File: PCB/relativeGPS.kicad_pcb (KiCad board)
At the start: 2 copper layers, 60 x 60 mm, 90 parts, among them CN1 FTSH-107-01-L-DV-K-P-TR, CN2 Solder_Jumper-2_Open, CN3 TC2030-IDC, CN4 5033981892, IC1 MIC5330-SSYML-TR, SW1 switch_slide_2pos, SW2 EVQ-P7A01P, SW3 EVQ-P7A01P, U1 LSM303AH, U10 RYLR998, U11 74LVC1T45GW,125, U2 TCA39306DCUR, U3 BGA725L6E6327FTSA1, U4 ST1S12GR, U5 B39162B4327P810, U6 TESEO-LIV3R, U7 AAA_2X_Holder, U8 TPS61222DCKR, U9 TPS79318DBVR

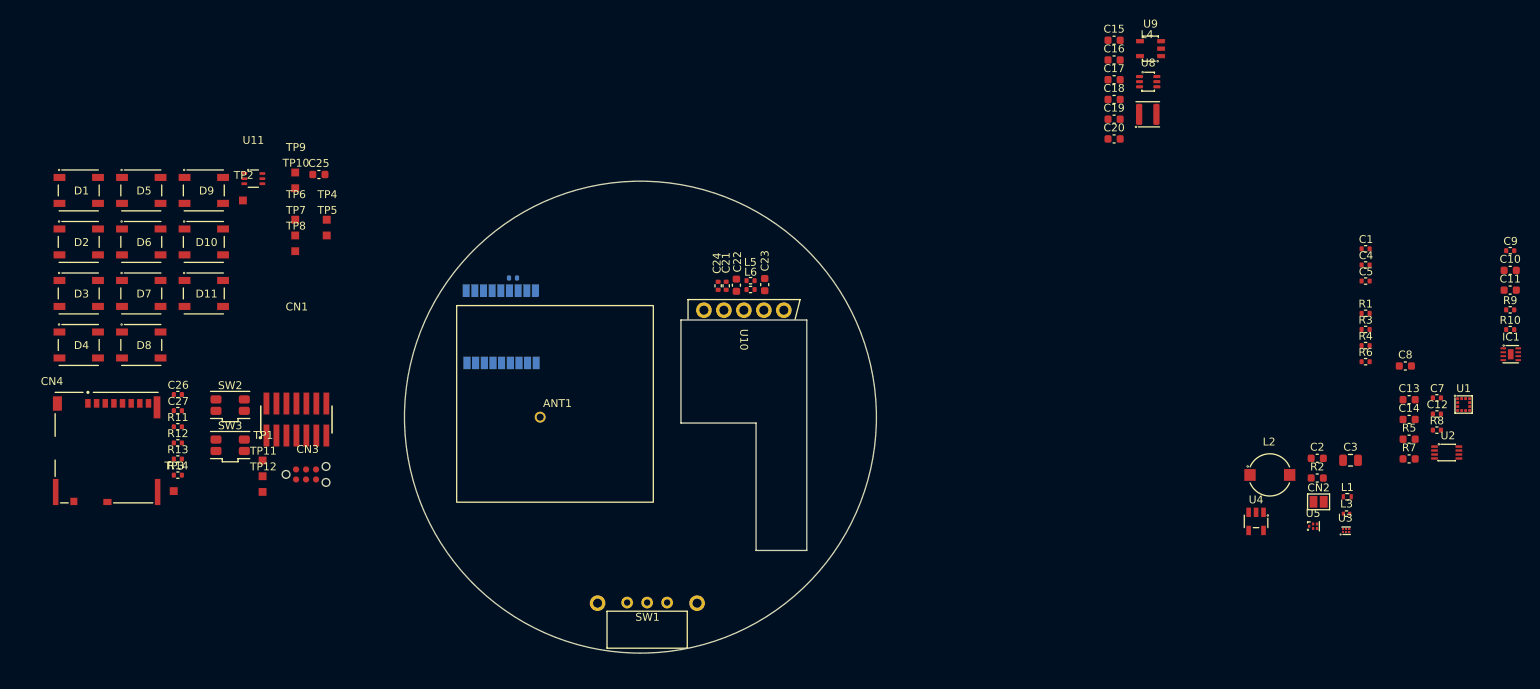
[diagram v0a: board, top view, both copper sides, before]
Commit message: Layout start
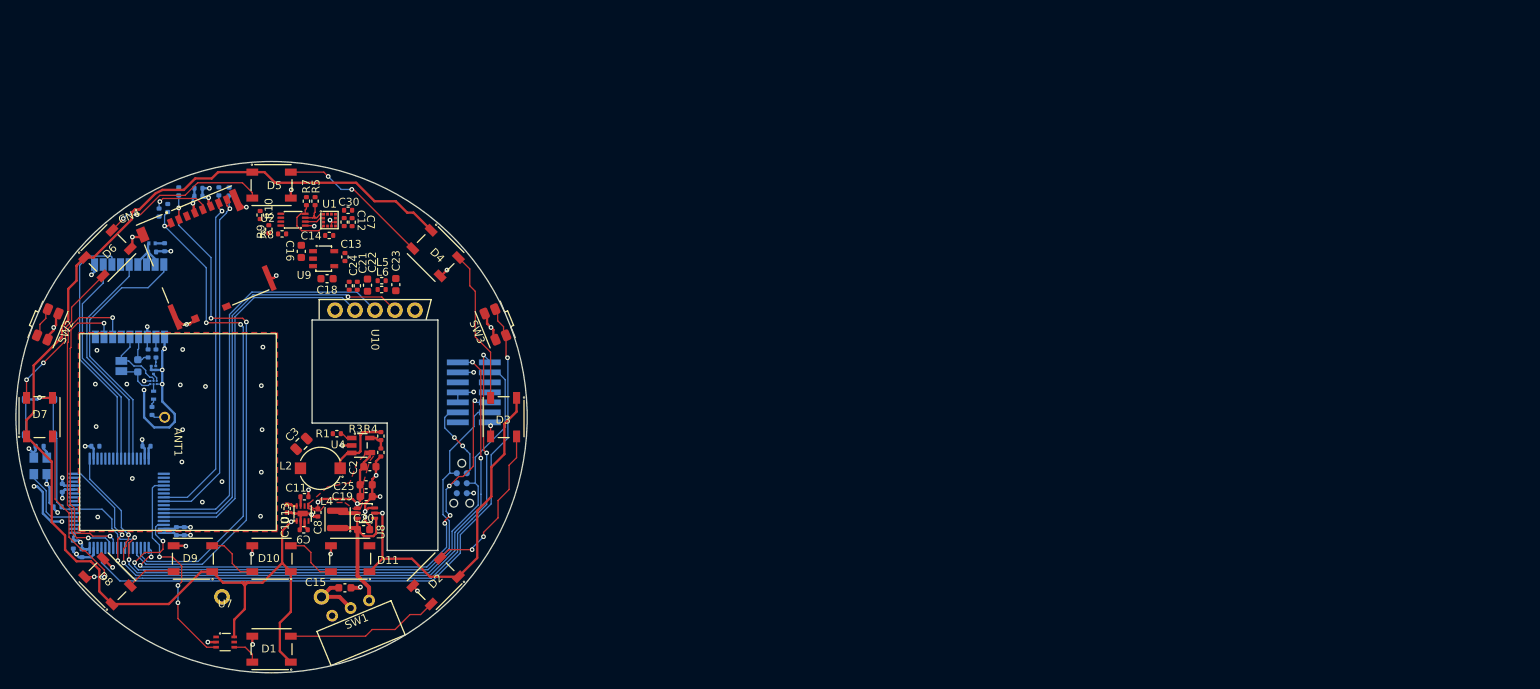
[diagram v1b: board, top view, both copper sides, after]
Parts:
- removed IC1: MIC5330-SSYML-TR, 004-Power:MIC5330
- removed TP1, TP10, TP11, TP12, TP2, TP3, TP4, TP5, TP6, TP7, TP8, TP9: TP_square_1mm, 011-Misc:Testpoint_square_1mm
- added B7: AAA_2X_Holder, 004-Power:AAA_2X_Holder, B.Cu at (100.0, 99.2)
- added C28: C_10nF_50V_10%_X7R_0402_H0.55, 002-Capacitors:C_0402_H0.55, B.Cu at (70.5, 103.7)
- added C29: C_100nF_50V_10%_X7R_0402_H0.55, 002-Capacitors:C_0402_H0.55, B.Cu at (72.8, 111.4)
- added C30: C_2.2uF_25V_25%_X5R_0402_H0.55, 002-Capacitors:C_0402_H0.55, F.Cu at (109.7, 73.7)
- added C31: C_100nF_50V_10%_X7R_0402_H0.55, 002-Capacitors:C_0402_H0.55, B.Cu at (74.8, 116.2)
- added C32: C_100nF_50V_10%_X7R_0402_H0.55, 002-Capacitors:C_0402_H0.55, B.Cu at (73.4, 109.0)
- added C33: C_100nF_50V_10%_X7R_0402_H0.55, 002-Capacitors:C_0402_H0.55, B.Cu at (77.6, 103.7)
- added C34: C_100nF_50V_10%_X7R_0402_H0.55, 002-Capacitors:C_0402_H0.55, B.Cu at (84.1, 103.7)
- added C35: C_100nF_50V_10%_X7R_0402_H0.55, 002-Capacitors:C_0402_H0.55, B.Cu at (87.9, 114.5)
- added C36: C_10uF_10V_20%_X5R_0402_H0.55, 002-Capacitors:C_0402_H0.55, B.Cu at (88.9, 114.5)
- added R15: R_0R_1%_1/16W_0402, 001-Resistors:R_0402_H0.4, B.Cu at (85.7, 74.0)
- added SW4: TL3315NF160Q, 009-Connectors:TL3315NF160Q, B.Cu at (70.5, 100.0)
- added U12: ASE-8.000MHZ-L-C-T, 005-ICs:ASE-8.000MHZ-L-C-T, B.Cu at (70.6, 106.2)
- added U13: MIC5330-SSYML-TR, 004-Power:MIC5330, F.Cu at (103.9, 112.3)
- C1, C26, C27, C4, C5, CN1, CN2, CN3, L1, L3, R11, R12, R13, R14, R2, R6, U3, U5: moved to B.Cu
- C10, C11, C8: value C_1uF_50V_10%_X5R_0603_H0.9 -> C_1uF_50V_10%_X5R_0402_H0.55; footprint 002-Capacitors:C_0603_H0.95 -> 002-Capacitors:C_0402_H0.55
- C13: value C_220nF_50V_10%_X7R_0603_H0.9 -> C_2.2uF_25V_25%_X5R_0402_H0.55; footprint 002-Capacitors:C_0603_H0.95 -> 002-Capacitors:C_0402_H0.55
- C14: value C_10uF_10V_20%_X5R_0603H0.9 -> C_220nF_16V_10%_X7R_0402_H0.55; footprint 002-Capacitors:C_0603_H0.95 -> 002-Capacitors:C_0402_H0.55
- C17: value C_10uF_10V_20%_X5R_0603H0.9 -> C_100nF_50V_10%_X7R_0402_H0.55; footprint 002-Capacitors:C_0603_H0.95 -> 002-Capacitors:C_0402_H0.55; moved to B.Cu
- R5, R7: value R_4k7_1%_1/10W_0603 -> R_4k7_5%_1/16W_0402; footprint 001-Resistors:R_0603_H0.55 -> 001-Resistors:R_0402_H0.4
- U11: value 74LVC1T45GW,125 -> STM32L431RCT6TR; footprint 005-ICs:TSSOP6_SOT363-2.step -> 007-MCUs:LQFP-64_10x10mm_P0.5mm; moved to B.Cu
- U7: value AAA_2X_Holder -> 74LVC1T45GW.125; footprint 004-Power:AAA_2X_Holder -> 005-ICs:TSSOP6_SOT363-2.step; moved to F.Cu
- moved R9 159.4 mm to (98.5, 74.3), turned to -90 degrees
- moved C10 158.4 mm to (102.0, 111.6), turned to -90 degrees
- moved R10 158.3 mm to (99.7, 76.1), turned to 90 degrees
- moved C9 157.4 mm to (104.1, 114.3), turned to 180 degrees
- moved L3 155.7 mm to (84.8, 77.9), turned to 180 degrees
- moved C1 155.7 mm to (84.8, 99.2), turned to 90 degrees
- moved C11 155.5 mm to (104.2, 110.1)
- moved R6 154.8 mm to (84.3, 91.9), turned to 90 degrees
- moved C4 154.2 mm to (85.3, 91.9), turned to 90 degrees
- moved CN2 153.2 mm to (80.9, 93.5), turned to -90 degrees
- moved U3 152.8 mm to (85.0, 95.6)
- moved C5 152.8 mm to (86.4, 78.4), turned to -90 degrees
- moved L1 152.3 mm to (85.0, 97.2), turned to 90 degrees
- moved R2 150.6 mm to (83.0, 93.5), turned to 90 degrees
- moved U2 149.6 mm to (102.7, 74.9), turned to 180 degrees
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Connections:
- C11 pad 1: +3.3V -> +3.3V_LORA
- C13 pad 1: Net-(U1-C1) -> +1V8
- C14 pad 1: +1V8 -> Net-(U1-C1)
- C15 pad 1: +3V8 -> +BATT
- C16 pad 1: +3V8 -> +3V0
- C17 pad 1: +1V8 -> +3.3V
- C20 pad 1: +3V8 -> +3V0
- C23 pad 1: +3.3V -> +3.3V_LORA
- C3 pad 1: +3.3V -> +3.3V_GPS
- C5 pad 1: +3.3V -> +3.3V_GPS
- CN3 pad 6: /SWO -> unconnected-(CN3-SWO-Pad6)
- CN4 pad 5: /SD_CLK -> Net-(CN4-CLK)
- L2 pad 2: +3.3V -> +3.3V_GPS
- L3 pad 1: +3.3V -> +3.3V_GPS
- L4 pad 1: +3V8 -> +3V0
- L5 pad 1: +3.3V -> +3.3V_LORA
- SW1 pad 1: +3V8 -> unconnected-(SW1-Pad1)
- SW1 pad 2: +3V8 -> +BATT
- SW1 pad 3: unconnected-(SW1-Pad3) -> +3V0
- U11 pad 1: +3V3 -> +3.3V
- U11 pad 2: GND -> unconnected-(U11-PC13-Pad2)
- U11 pad 3: /LED_DATA -> unconnected-(U11-PC14-OSC32_IN-Pad3)
- U11 pad 4: Net-(D1-DIN) -> unconnected-(U11-PC15-OSC32_OUT-Pad4)
- U11 pad 5: +3V3 -> Net-(U11-PH0-OSC_IN)
- U11 pad 6: +5V -> unconnected-(U11-PH1-OSC_OUT-Pad6)
- U7 pad 1: +3V8 -> +3V3
- U8 pad 1: +3V8 -> +3V0
- U8 pad 6: +3V8 -> +3V0
- U9 pad 1: +3V8 -> +3V0
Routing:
- net +5V: track 0.00 -> 227.8 mm, vias 0 -> 4
- net GND: track 0.00 -> 129.8 mm, vias 0 -> 67
- net /NRST: track 0.00 -> 100.7 mm, vias 0 -> 2
- net /UART_TX: track 0.00 -> 87.9 mm, vias 0 -> 4
- net /UART_RX: track 0.00 -> 87.3 mm, vias 0 -> 4
- net /BUTTON_2: track 0.00 -> 84.1 mm, vias 0 -> 1
- net /SWDIO: track 0.00 -> 72.5 mm, vias 0 -> 2
- net /SWCLK: track 0.00 -> 67.4 mm, vias 0 -> 6
- net /SD_DAT3: track 0.00 -> 66.3 mm, vias 0 -> 3
- net /SD_DAT2: track 0.00 -> 63.0 mm, vias 0 -> 3
- net /RYLR998_TX: track 0.00 -> 55.2 mm, vias 0 -> 1
- net /RYLR998_RX: track 0.00 -> 52.7 mm
- net /RYLR998_NRST: track 0.00 -> 50.1 mm
- net /SD_DAT1: track 0.00 -> 45.8 mm, vias 0 -> 1
- net /SD_DAT0: track 0.00 -> 44.6 mm, vias 0 -> 1
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- added copper zone on F.Cu, net +5V
- added copper zone on F.Cu, net GND
- added copper zone on In1.Cu, net GND
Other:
- board size 60 x 60 mm -> 65 x 65 mm
- copper layers 2 -> 4
